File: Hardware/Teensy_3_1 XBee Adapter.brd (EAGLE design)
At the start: 27.9 x 86.4 mm, 34 parts

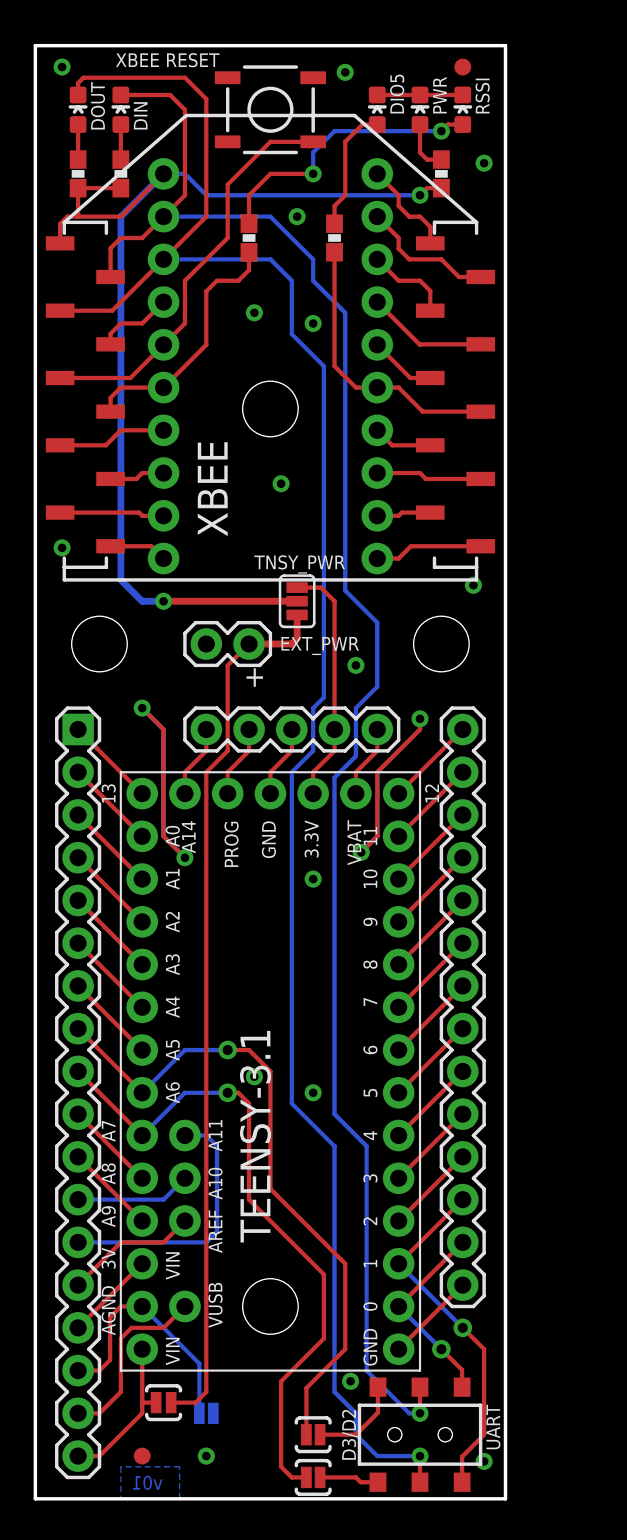
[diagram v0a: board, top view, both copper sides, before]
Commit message: Opened the board up a bit
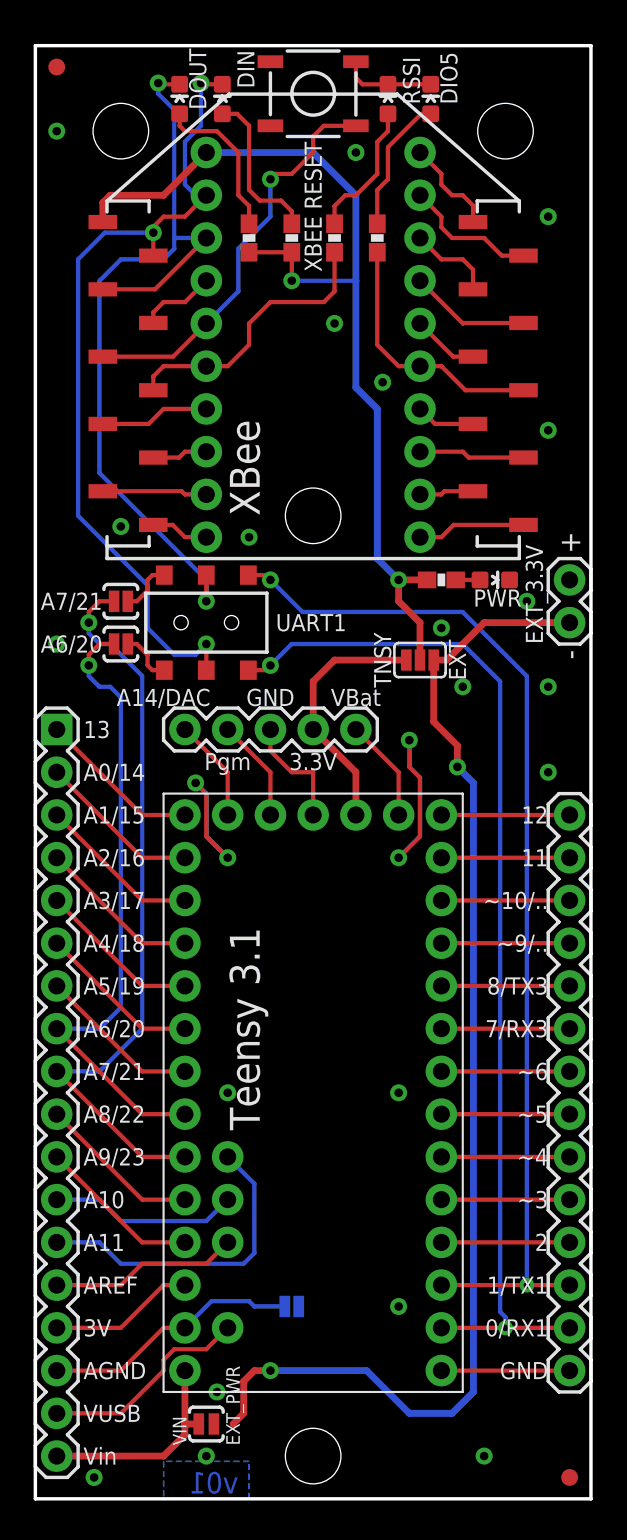
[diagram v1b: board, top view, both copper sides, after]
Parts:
- removed EXT_PWR: M02PTH, SparkFun-Connectors:1X02
- added EXT_3.3V: M02PTH, SparkFun-Connectors:1X02
- JP1: value TEENSY-3.1 -> TEENSY-3.1NOSILK; device Testing:TEENSY-3.1 -> Testing:TEENSY-3.1_NOSILK
- LOGO2: value OSHW-LOGOS -> OSHW-LOGOM; device SparkFun-Aesthetics:OSHW-LOGO-S -> SparkFun-Aesthetics:OSHW-LOGO-M
- LOGO3: value SFE_LOGO_NAME_FLAME.1_INCH -> SFE_LOGO_NAME_FLAME.2_INCH; device SparkFun-Aesthetics:SFE_LOGO_NAME_FLAME_.1 -> SparkFun-Aesthetics:SFE_LOGO_NAME_FLAME_.2
- moved SJ1 53.3 mm to (5.08, 53.3)
- moved S2 49.9 mm to (10.2, 52.1)
- moved SJ3 48.4 mm to (5.08, 50.8)
- moved STANDOFF1 30.7 mm to (27.9, 81.3)
- moved STANDOFF2 30.5 mm to (5.08, 81.3)
- moved LED1 28.3 mm to (27.3, 54.6), turned to 270 degrees
- moved FID2 25.4 mm to (31.8, 1.27)
- moved FID1 24.1 mm to (1.27, 85.1)
- moved R11 24.1 mm to (24.1, 54.6), turned to 180 degrees
- moved LOGO2 16.6 mm to (21.6, 3.49)
- moved FRAME1 11.4 mm to (-17.8, -11.4)
- moved R1 10.9 mm to (15.2, 74.9)
- moved R3 10.9 mm to (12.7, 74.9)
- moved LOGO3 10.2 mm to (12.4, 14.6)
- moved STANDOFF3 9.25 mm to (16.5, 2.54)
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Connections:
- removed net EXT_PWR: EXT_PWR.2, SJ4.1, SJ5.2
- new net EXT_3.3V: EXT_3.3V.2, SJ4.1, SJ5.2
- net GND: now also EXT_3.3V.1; no longer EXT_PWR.1
- net IN: now also S2.5; no longer S2.2
- net N$140: now also S2.6; no longer S2.3
- net N$141: now also S2.3; no longer S2.6
- net OUT: now also S2.2; no longer S2.5
- net UART_RX: now also S2.1; no longer S2.4
- net UART_TX: now also S2.4; no longer S2.1
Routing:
- net EXT_3.3V: track 0.00 -> 71.8 mm, vias 0 -> 2
- net IN: track 112.8 -> 49.3 mm, vias 1 -> 2
- net EXT_PWR: track 52.3 -> 0.00 mm
- net OUT: track 101.9 -> 50.0 mm, vias 1 -> 3
- net UART_RX: track 11.7 -> 62.7 mm, vias 1 -> 2
- net UART_TX: track 21.0 -> 62.9 mm, vias 1 -> 2
- net N$43: track 17.3 -> 8.22 mm, vias 2 -> 0
- net XBEE_VDD: track 66.2 -> 57.4 mm
- net N$17: track 2.08 -> 9.50 mm
- net GND: track 56.9 -> 49.5 mm, vias 20 -> 25
- net N$19: track 2.08 -> 9.35 mm
- net A7/21: track 39.3 -> 44.1 mm
- net A5/19/SCL0: track 5.39 -> 9.72 mm
- net A9/23: track 5.39 -> 9.72 mm
- net A4/18/SDA0: track 5.39 -> 9.72 mm
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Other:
- board size 27.9 x 86.4 mm -> 33 x 86.4 mm
- board text added: "-"
- board text added: "0/RX1"
- board text added: "1/TX1"
- board text added: "11"
- board text added: "12"
- board text added: "13"
- board text added: "2"
- board text added: "3.3V"
- board text added: "3V"
- board text added: "7/RX3"
- board text added: "8/TX3"
- board text added: "A0/14"
- board text added: "A1/15"
- board text added: "A10"
- board text added: "A11"
- board text added: "A14/DAC"
- board text added: "A2/16"
- board text added: "A3/17"
- board text added: "A4/18"
- board text added: "A5/19"
- board text added: "A6/20"
- board text added: "A7/21"
- board text added: "A8/22"
- board text added: "A9/23"
- board text added: "AGND"
- board text added: "AREF"
- board text added: "DGND"
- board text added: "EXT"
- board text added: "EXT_PWR"
- board text added: "Pgm"
- board text added: "TNSY"
- board text added: "Teensy 3.1"
- board text added: "UART1"
- board text added: "VBat"
- board text added: "VIN"
- board text added: "VUSB"
- board text added: "Vin"
- board text added: "XBee"
- board text added: "~10/.."
- board text added: "~3"
- board text added: "~4"
- board text added: "~5"
- board text added: "~6"
- board text added: "~9/.."
- board text removed: "D3/D2"
- board text removed: "TNSY_PWR"
- board text removed: "UART"
- board text removed: "XBEE"
